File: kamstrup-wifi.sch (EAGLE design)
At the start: 20 parts, among them T1 BT137, T2 BT137, U1 ESP8266-07

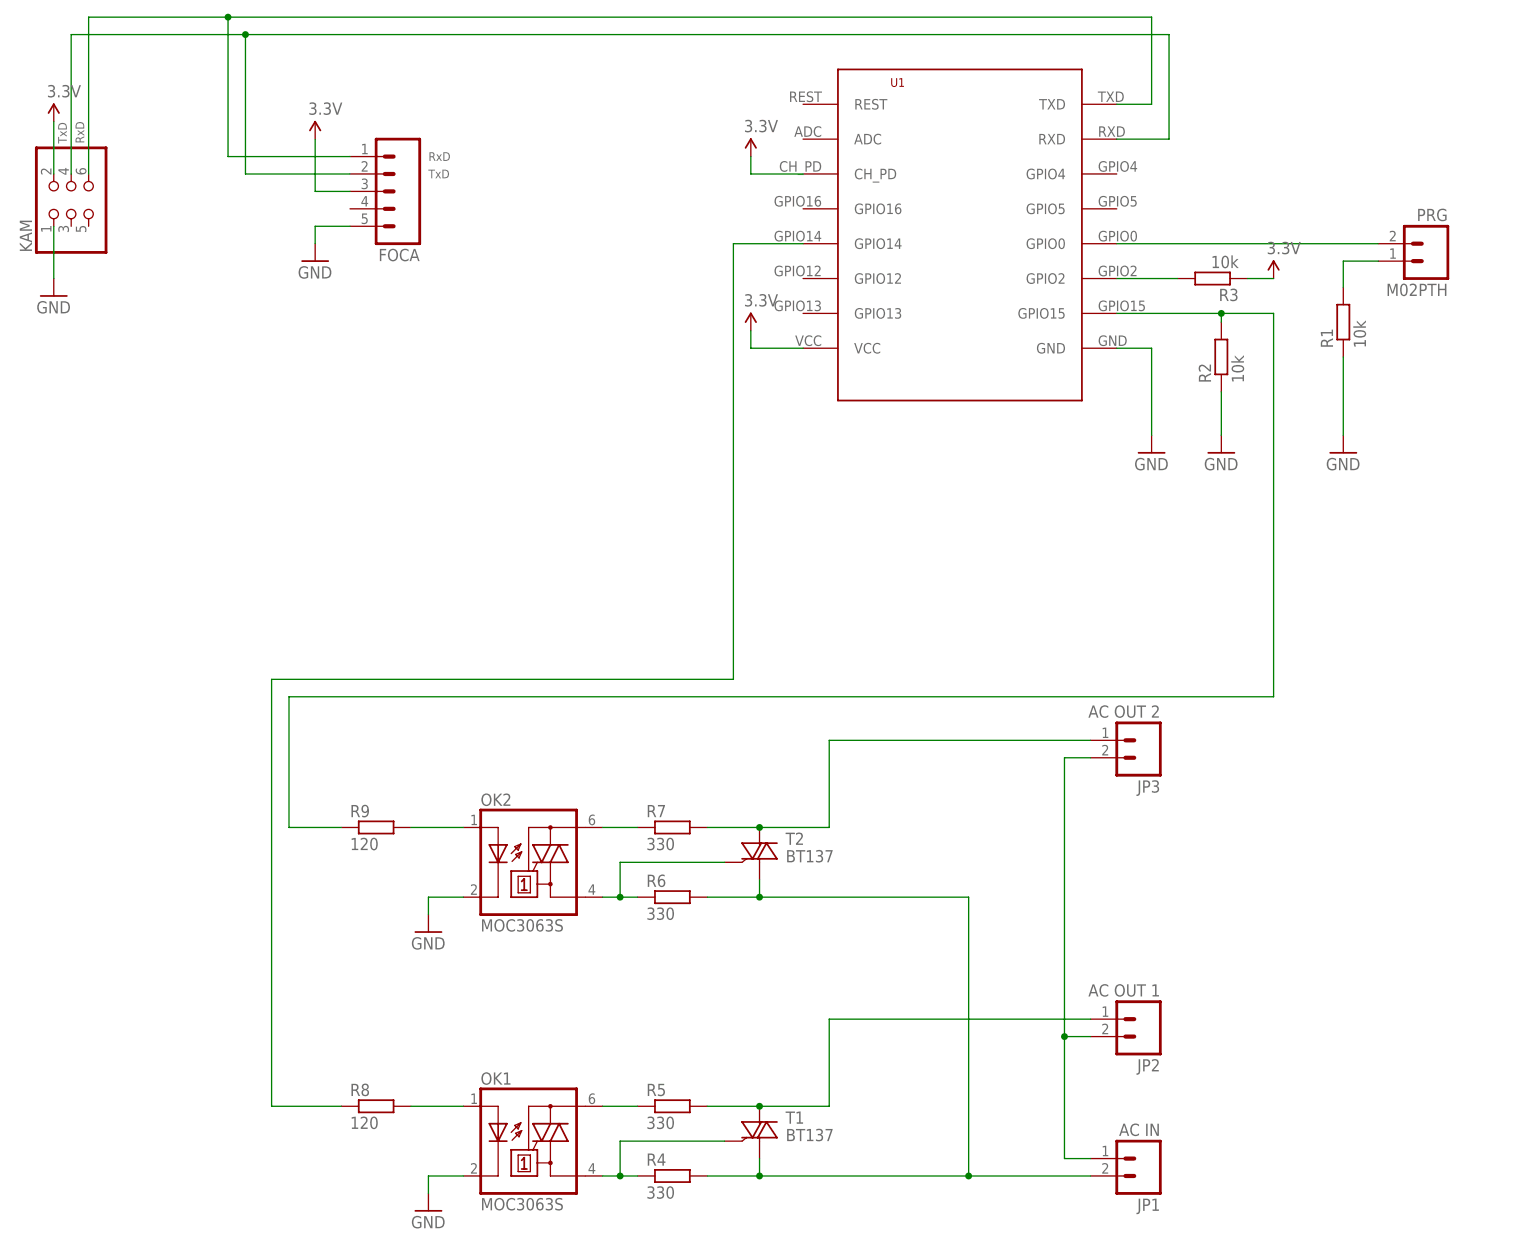
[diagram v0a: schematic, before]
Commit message: Sdcard
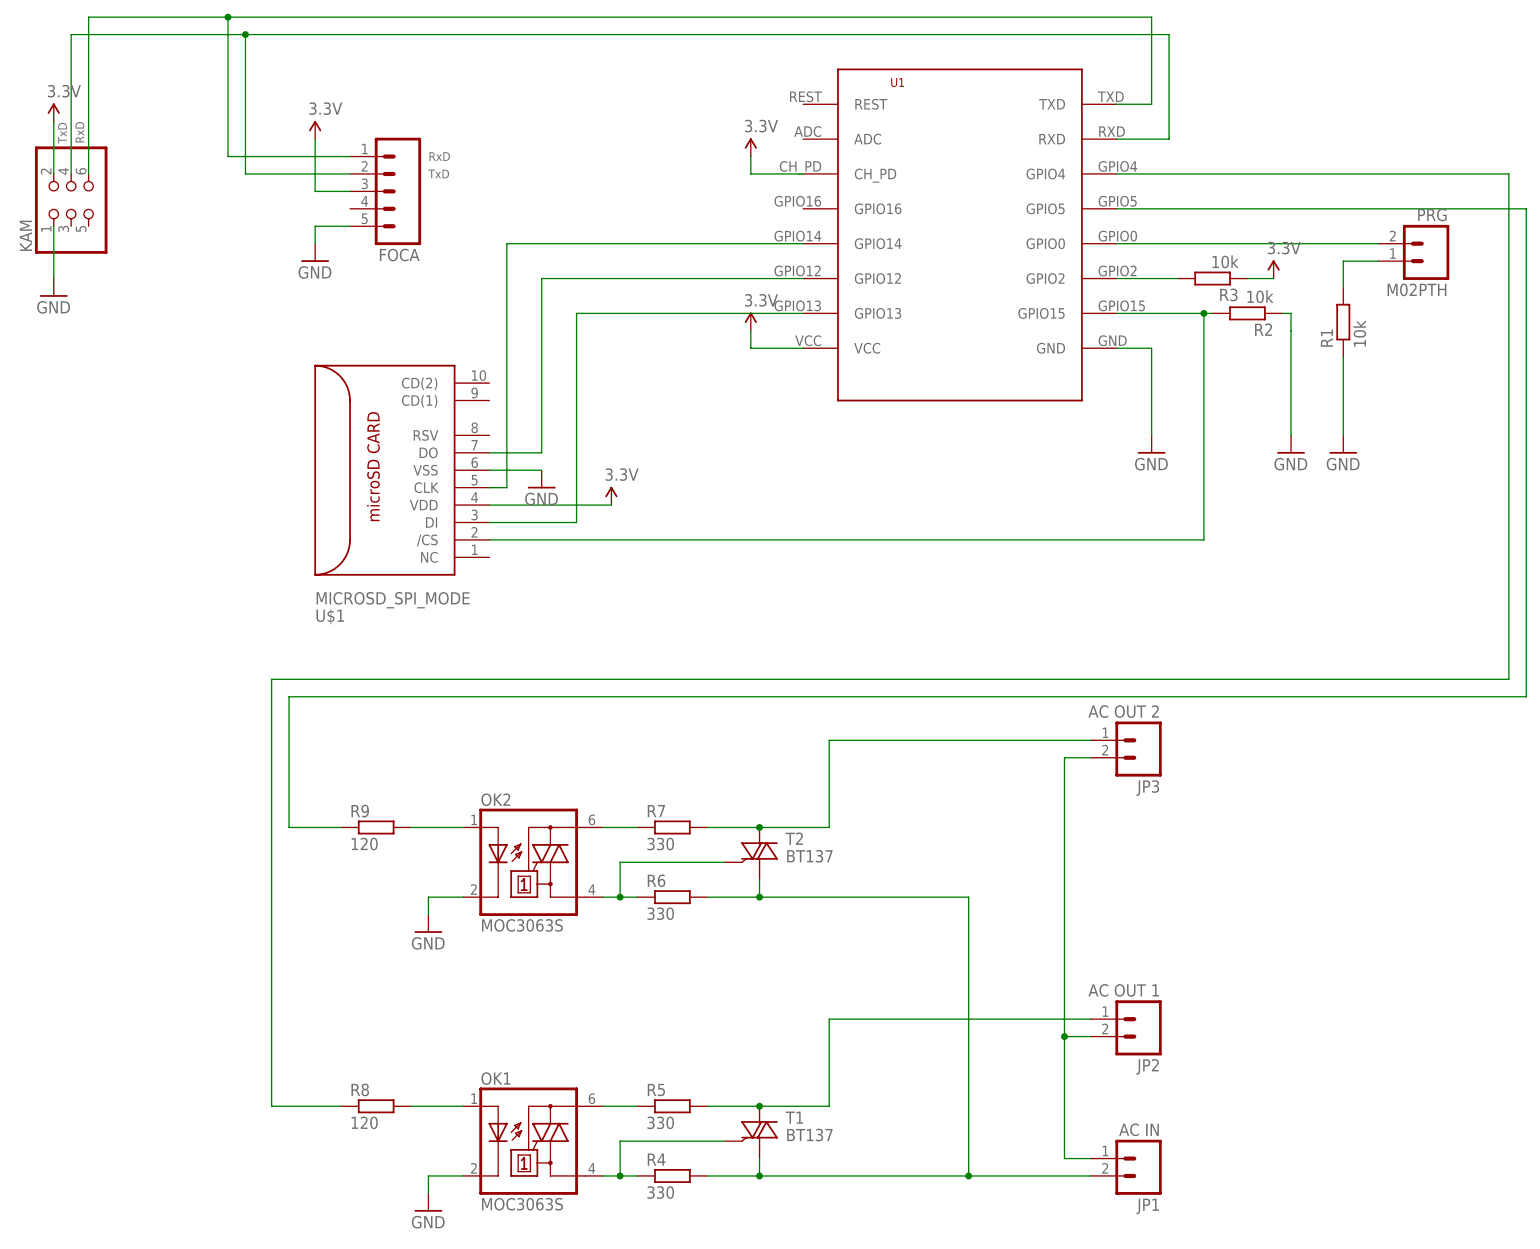
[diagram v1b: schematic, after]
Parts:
- added U$1: MICROSD_SPI_MODE, con-molex-microsd:MICROSD_SPI_MODE
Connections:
- new net N$10: U$1.DO, U1.GPIO12
- new net N$17: U$1.DI, U1.GPIO13
- new net N$19: U$1.CLK, U1.GPIO14
- new net N$20: R2.2, U$1./CS, U1.GPIO15
- net 3.3V: now also U$1.VDD
- net GND: now also U$1.VSS
- net N$11: now also U1.GPIO4; no longer U1.GPIO14
- net N$16: now also U1.GPIO5; no longer R2.2, U1.GPIO15
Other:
- moved on the sheet: R2
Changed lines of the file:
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@@
 <?xml version="1.0" encoding="utf-8"?>
 <!DOCTYPE eagle SYSTEM "eagle.dtd">
-<eagle version="8.4.0">
+<eagle version="9.0.1">
 <drawing>
 <settings>
-<setting alwaysvectorfont="yes"/>
+<setting alwaysvectorfont="no"/>
 <setting keepoldvectorfont="yes"/>
 <setting verticaltext="up"/>
 </settings>
-<grid distance="0.1" unitdist="inch" unit="inch" style="lines" multiple="1" display="no" altdistance="0.01" altunitdist="inch" altunit="inch"/>
+<grid distance="0.05" unitdist="inch" unit="inch" style="lines" multiple="1" display="no" altdistance="0.005" altunitdist="inch" altunit="inch"/>
 <layers>
 <layer number="1" name="Top" color="4" fill="1" visible="no" active="no"/>
@@
 <part name="SUPPLY5" library="SparkFun-Aesthetics" deviceset="3.3V" device=""/>
 <part name="R3" library="rcl" deviceset="R-EU_" device="R0805" value="10k"/>
+<part name="U$1" library="con-molex-microsd" deviceset="MICROSD_SPI_MODE" device=""/>
+<part name="GND7" library="SparkFun-Aesthetics" deviceset="GND" device=""/>
+<part name="SUPPLY3" library="SparkFun-Aesthetics" deviceset="3.3V" device=""/>
 </parts>
 <sheets>
@@
 <instance part="SUPPLY2" gate="G$1" x="78.74" y="71.12"/>
 <instance part="SUPPLY7" gate="G$1" x="78.74" y="45.72"/>
-<instance part="R2" gate="G$1" x="147.32" y="41.91" rot="R90"/>
-<instance part="GND3" gate="1" x="147.32" y="27.94"/>
+<instance part="R2" gate="G$1" x="151.13" y="48.26" rot="R180"/>
+<instance part="GND3" gate="1" x="157.48" y="27.94"/>
 <instance part="SUPPLY5" gate="G$1" x="154.94" y="53.34"/>
 <instance part="R3" gate="G$1" x="146.05" y="53.34" rot="R180"/>
+<instance part="U$1" gate="G$1" x="27.94" y="25.4" rot="MR180"/>
+<instance part="GND7" gate="1" x="48.26" y="22.86"/>
+<instance part="SUPPLY3" gate="G$1" x="58.42" y="20.32"/>
 </instances>
 <busses>
@@
 <pinref part="GND3" gate="1" pin="GND"/>
 <pinref part="R2" gate="G$1" pin="1"/>
-<wire x1="147.32" y1="30.48" x2="147.32" y2="36.83" width="0.1524" layer="91"/>
+<wire x1="157.48" y1="30.48" x2="157.48" y2="45.72" width="0.1524" layer="91"/>
+<wire x1="157.48" y1="45.72" x2="157.48" y2="48.26" width="0.1524" layer="91"/>
+<wire x1="157.48" y1="48.26" x2="156.21" y2="48.26" width="0.1524" layer="91"/>
+</segment>
+<segment>
+<pinref part="U$1" gate="G$1" pin="VSS"/>
+<pinref part="GND7" gate="1" pin="GND"/>
+<wire x1="40.64" y1="25.4" x2="48.26" y2="25.4" width="0.1524" layer="91"/>
 </segment>
 </net>
@@
 <pinref part="SUPPLY5" gate="G$1" pin="3.3V"/>
 <wire x1="151.13" y1="53.34" x2="154.94" y2="53.34" width="0.1524" layer="91"/>
+</segment>
+<segment>
+<pinref part="U$1" gate="G$1" pin="VDD"/>
+<pinref part="SUPPLY3" gate="G$1" pin="3.3V"/>
+<wire x1="40.64" y1="20.32" x2="58.42" y2="20.32" width="0.1524" layer="91"/>
 </segment>
 </net>
@@
 <net name="N$11" class="0">
 <segment>
-<wire x1="76.2" y1="-5.08" x2="76.2" y2="58.42" width="0.1524" layer="91"/>
-<pinref part="U1" gate="G$1" pin="GPIO14"/>
-<wire x1="76.2" y1="58.42" x2="86.36" y2="58.42" width="0.1524" layer="91"/>
-<wire x1="76.2" y1="-5.08" x2="8.89" y2="-5.08" width="0.1524" layer="91"/>
 <wire x1="8.89" y1="-5.08" x2="8.89" y2="-67.31" width="0.1524" layer="91"/>
 <pinref part="R8" gate="G$1" pin="1"/>
 <wire x1="8.89" y1="-67.31" x2="19.05" y2="-67.31" width="0.1524" layer="91"/>
+<wire x1="8.89" y1="-5.08" x2="189.23" y2="-5.08" width="0.1524" layer="91"/>
+<pinref part="U1" gate="G$1" pin="GPIO4"/>
+<wire x1="189.23" y1="-5.08" x2="189.23" y2="68.58" width="0.1524" layer="91"/>
+<wire x1="189.23" y1="68.58" x2="132.08" y2="68.58" width="0.1524" layer="91"/>
 </segment>
 </net>
 <net name="N$16" class="0">
 <segment>
-<wire x1="154.94" y1="-7.62" x2="154.94" y2="48.26" width="0.1524" layer="91"/>
-<pinref part="U1" gate="G$1" pin="GPIO15"/>
-<wire x1="154.94" y1="48.26" x2="147.32" y2="48.26" width="0.1524" layer="91"/>
-<pinref part="R2" gate="G$1" pin="2"/>
-<wire x1="147.32" y1="48.26" x2="132.08" y2="48.26" width="0.1524" layer="91"/>
-<wire x1="147.32" y1="46.99" x2="147.32" y2="48.26" width="0.1524" layer="91"/>
-<junction x="147.32" y="48.26"/>
 <pinref part="R9" gate="G$1" pin="1"/>
 <wire x1="11.43" y1="-26.67" x2="19.05" y2="-26.67" width="0.1524" layer="91"/>
-<wire x1="154.94" y1="-7.62" x2="11.43" y2="-7.62" width="0.1524" layer="91"/>
 <wire x1="11.43" y1="-7.62" x2="11.43" y2="-26.67" width="0.1524" layer="91"/>
+<wire x1="11.43" y1="-7.62" x2="191.77" y2="-7.62" width="0.1524" layer="91"/>
+<pinref part="U1" gate="G$1" pin="GPIO5"/>
+<wire x1="191.77" y1="-7.62" x2="191.77" y2="63.5" width="0.1524" layer="91"/>
+<wire x1="191.77" y1="63.5" x2="132.08" y2="63.5" width="0.1524" layer="91"/>
 </segment>
 </net>
@@
 </segment>
 </net>
+<net name="N$10" class="0">
+<segment>
+<pinref part="U1" gate="G$1" pin="GPIO12"/>
+<wire x1="86.36" y1="53.34" x2="48.26" y2="53.34" width="0.1524" layer="91"/>
+<wire x1="48.26" y1="53.34" x2="48.26" y2="27.94" width="0.1524" layer="91"/>
+<pinref part="U$1" gate="G$1" pin="DO"/>
+<wire x1="48.26" y1="27.94" x2="40.64" y2="27.94" width="0.1524" layer="91"/>
+</segment>
+</net>
+<net name="N$17" class="0">
+<segment>
+<pinref part="U$1" gate="G$1" pin="DI"/>
+<wire x1="40.64" y1="17.78" x2="53.34" y2="17.78" width="0.1524" layer="91"/>
+<wire x1="53.34" y1="17.78" x2="53.34" y2="48.26" width="0.1524" layer="91"/>
+<pinref part="U1" gate="G$1" pin="GPIO13"/>
+<wire x1="53.34" y1="48.26" x2="86.36" y2="48.26" width="0.1524" layer="91"/>
+</segment>
+</net>
+<net name="N$19" class="0">
+<segment>
+<pinref part="U1" gate="G$1" pin="GPIO14"/>
+<wire x1="86.36" y1="58.42" x2="43.18" y2="58.42" width="0.1524" layer="91"/>
+<wire x1="43.18" y1="58.42" x2="43.18" y2="22.86" width="0.1524" layer="91"/>
+<pinref part="U$1" gate="G$1" pin="CLK"/>
+<wire x1="43.18" y1="22.86" x2="40.64" y2="22.86" width="0.1524" layer="91"/>
+</segment>
+</net>
+<net name="N$20" class="0">
+<segment>
+<pinref part="U1" gate="G$1" pin="GPIO15"/>
+<pinref part="R2" gate="G$1" pin="2"/>
+<wire x1="146.05" y1="48.26" x2="144.78" y2="48.26" width="0.1524" layer="91"/>
+<pinref part="U$1" gate="G$1" pin="/CS"/>
+<wire x1="144.78" y1="48.26" x2="132.08" y2="48.26" width="0.1524" layer="91"/>
+<wire x1="40.64" y1="15.24" x2="144.78" y2="15.24" width="0.1524" layer="91"/>
+<wire x1="144.78" y1="15.24" x2="144.78" y2="48.26" width="0.1524" layer="91"/>
+<junction x="144.78" y="48.26"/>
+</segment>
+</net>
